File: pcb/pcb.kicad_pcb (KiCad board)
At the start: 4 copper layers, 71.5 x 115.4 mm, 173 parts, among them J1 AudioJack3_SwitchTR, J100 Conn_02x05_Odd_Even, J102 Conn_01x03, J500 FPC_18P_1.0MM, J600 USB_B_Micro, Q300 IRLML6402, SW1 SW_SP3T, SW700 SW_Push, SW701 SW_Push, SW702 SW_Push, SW703 SW_Push, SW704 SW_Push, SW705 SW_Push, SW706 SW_Push, SW707 SW_Push, U1 LTC3456, U100 LPC5500, U400 CS43130, U401 ADP150-3.0, U402 ADP150-1.8, U403 ADP150-1.8, U404 SN74AVC4T245PW, U405 PCA9306, U501 LT1617, U502 LM324, U600 USBLC6-2SC6, Y1 32.768kHz, Y2 24MHz, Y400 22.5792MHz

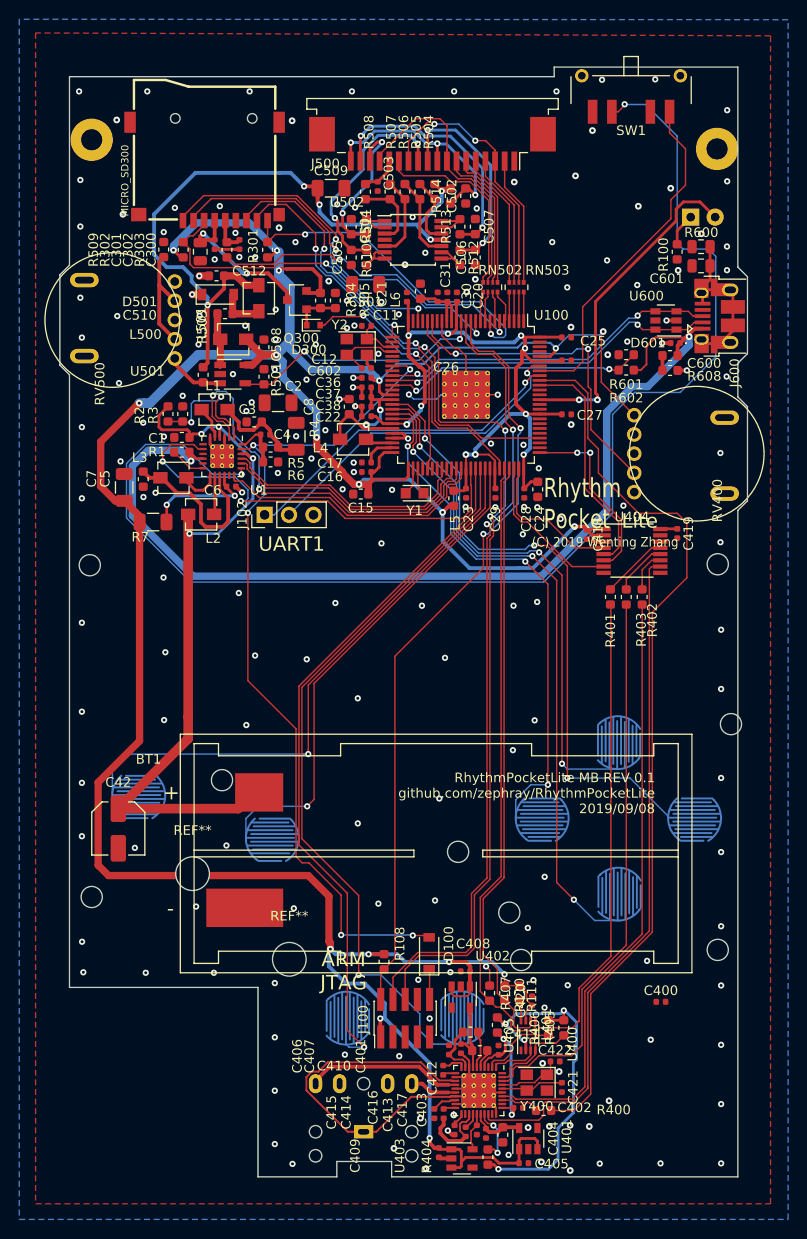
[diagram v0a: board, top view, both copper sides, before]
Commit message: rev 0.1
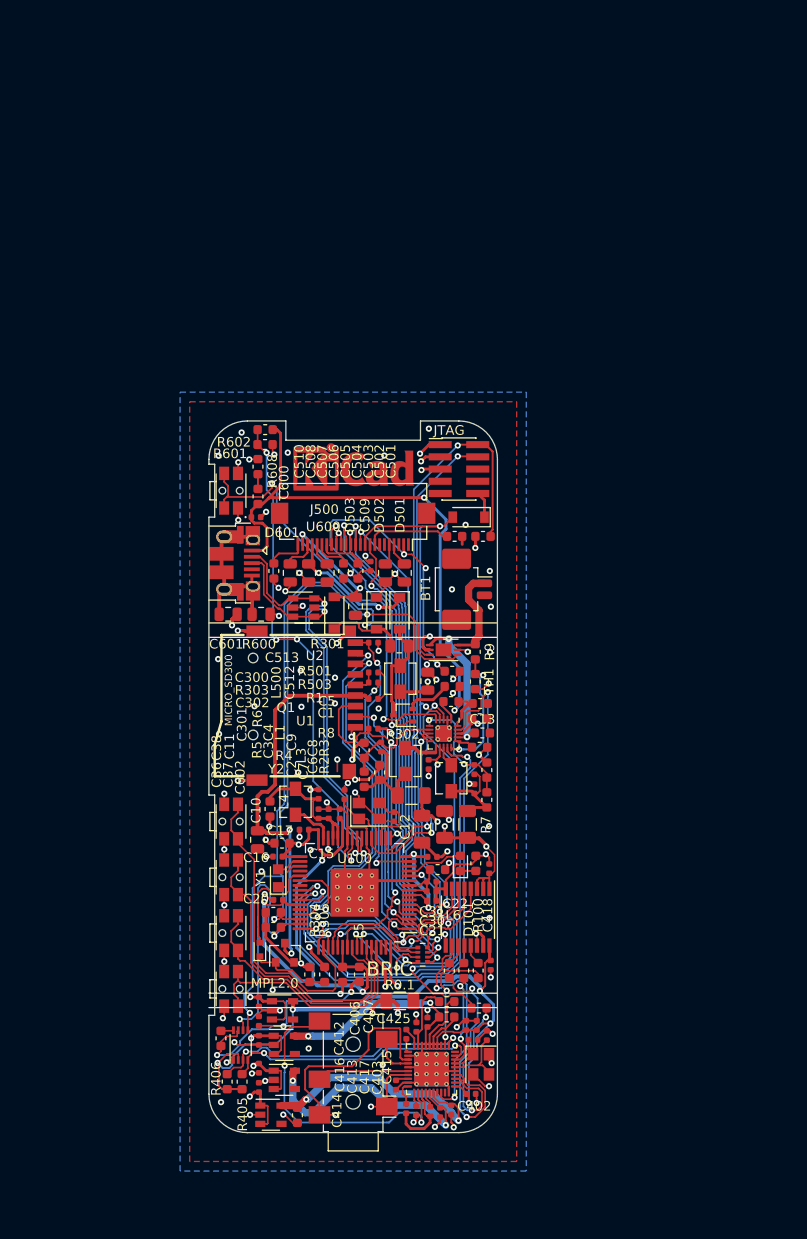
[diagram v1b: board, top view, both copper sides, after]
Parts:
- removed C23, C25, C26, C27, C28, C29: 100nF, Capacitor_SMD:C_0402_1005Metric
- removed C42: 100uF, Capacitor_SMD:C_Elec_5x5.4
- removed G***: LOGO, footprints:logo
- removed J102: Conn_01x03, Connector_PinHeader_2.54mm:PinHeader_1x03_P2.54mm_Vertical
- removed L2: 4.7uH, Inductor_SMD:L_Vishay_IHLP-1212
- removed L401: 120R, Inductor_SMD:L_0603_1608Metric
- removed L501: 22uH, Inductor_SMD:L_Vishay_IHLP-1212
- removed R404, R504, R505, R507, R508: 10K, Resistor_SMD:R_0603_1608Metric
- removed R506: 75K, Resistor_SMD:R_0603_1608Metric
- removed R509: 20K, Resistor_SMD:R_0603_1608Metric
- removed R510, R511, R512, R513, R514: 33, Resistor_SMD:R_0603_1608Metric
- removed the REF** at (128.3, 127.1)
- removed the REF** at (184.3, 111.5)
- removed the REF** at (182.8, 51.7)
- removed the REF** at (117.8, 50.8)
- removed the REF** at (131.4, 117.3)
- removed the REF** at (117.6, 95.0)
- removed the REF** at (138.4, 136.0)
- removed the REF** at (182.9, 94.9)
- removed the REF** at (117.8, 129.5)
- removed the REF** at (182.9, 135.0)
- removed the REF** at (155.9, 124.8)
- removed the REF** at (162.5, 136.1)
- removed the REF** at (161.2, 131.1)
- removed RN502: 33R, Resistor_SMD:R_Array_Convex_4x0402
- removed RV400: RK14J11A0A02, footprints:Potentiometer_RK14J
- removed RV500: RK14J11A0A02/50K, footprints:Potentiometer_RK14J
- removed SW700, SW705, SW706, SW707: SW_Push, footprints:contact
- removed U501: LT1617, Package_TO_SOT_SMD:TSOT-23-5
- removed U502: LM324, Package_SO:TSSOP-14_4.4x5mm_P0.65mm
- added C10: 22uF, Capacitor_SMD:C_0603_1608Metric, F.Cu at (136.3, 120.3)
- added C13: 10uF, Capacitor_SMD:C_0603_1608Metric, F.Cu at (158.4, 112.4)
- added C424: 1uF, Capacitor_SMD:C_0402_1005Metric, F.Cu at (135.2, 140.4)
- added C425: 100uF, Capacitor_SMD:C_1206_3216Metric, F.Cu at (149.8, 140.3)
- added C513: 4.7uF/25V, Capacitor_SMD:C_0805_2012Metric, F.Cu at (149.8, 103.4)
- added C9: 2.2uF, Capacitor_SMD:C_0402_1005Metric, F.Cu at (152.8, 115.7)
- added D502: MBR0530, Diode_SMD:D_SOD-123, F.Cu at (147.4, 100.0)
- added D503: MBR0530, Diode_SMD:D_SOD-123, F.Cu at (143.0, 99.9)
- added Q1: Q_NMOS_GSD, Package_TO_SOT_SMD:SOT-323_SC-70, F.Cu at (150.2, 110.6)
- added R502: 10K, Resistor_SMD:R_0603_1608Metric, F.Cu at (155.6, 92.0)
- added R8: 1.87K, Resistor_SMD:R_0603_1608Metric, F.Cu at (158.2, 113.9)
- added R9: 100K, Resistor_SMD:R_0603_1608Metric, F.Cu at (157.7, 104.0)
- added REF**: KiCad-Logo_5mm_SilkScreen, Symbol:KiCad-Logo_5mm_SilkScreen, B.Cu at (145.0, 147.4)
- added REF**: KiCad-Logo_5mm_Copper, Symbol:KiCad-Logo_5mm_Copper, F.Cu at (145.1, 85.3)
- added TH1: 100K, Resistor_SMD:R_0603_1608Metric, F.Cu at (157.7, 107.1)
- added U2: LTC2942-1, Package_DFN_QFN:DFN-6-1EP_3x2mm_P0.5mm_EP1.65x1.35mm, F.Cu at (154.4, 103.8)
- added U406: ADP150-1.8, Package_TO_SOT_SMD:SOT-23-5, F.Cu at (137.7, 141.3)
- BT1: value Battery -> Molex1.25; footprint footprints:BatteryHolder_Keystone_5204_5226 -> Connector_Molex:Molex_PicoBlade_53261-0271_1x02-1MP_P1.25mm_Horizontal
- C1: value 4.7uF -> 10uF
- C5: value 22uF -> 10uF
- C501, C509: value 22uF/25V -> 4.7uF/25V; footprint Capacitor_SMD:C_1206_3216Metric -> Capacitor_SMD:C_0805_2012Metric
- C502, C506, C507: value 4.7uF -> 4.7uF/25V; footprint Capacitor_SMD:C_0603_1608Metric -> Capacitor_SMD:C_0805_2012Metric
- C504, C505: value 4.7uF -> 1uF
- C508: value 10uF -> 4.7uF/25V; footprint Capacitor_SMD:C_0603_1608Metric -> Capacitor_SMD:C_0805_2012Metric
- C510: value 220nF -> 1uF
- C512: footprint Capacitor_SMD:C_0603_1608Metric -> Capacitor_SMD:C_0805_2012Metric
- C8: value 22uF -> 220pF; footprint Capacitor_SMD:C_0603_1608Metric -> Capacitor_SMD:C_0402_1005Metric
- D101: footprint LED_THT:LED_D5.0mm -> LED_SMD:LED_0603_1608Metric; moved to F.Cu
- J1: value AudioJack3_SwitchTR -> AudioJack3_SwitchDualS; footprint footprints:Jack_3.5mm_PJ307C -> footprints:Jack_3.5mm_PJ327E_5A; moved to F.Cu
- J500: value FPC_18P_1.0MM -> FH12A-24S-0.5SH; footprint Connector_FFC-FPC:TE_1-84953-8_1x18-1MP_P1.0mm_Horizontal -> Connector_FFC-FPC:Hirose_FH12-24S-0.5SH_1x24-1MP_P0.50mm_Horizontal
- L3: value 10uH -> 4.7uH
- L500: value 22uH -> 10uH
- R2: value 100K -> 2.05M
- R3: value 80.6K -> 649K
- R301, R302, R303: footprint Resistor_SMD:R_0603_1608Metric -> Resistor_SMD:R_0402_1005Metric
- R5: value 100K -> 1M
- R503: value 330K -> 3R
- SW1: value SW_SP3T -> SW_Push; footprint footprints:SW_SP3T_JSM0701SAQNL -> Button_Switch_SMD:SW_SPST_EVQP7C
- SW701, SW702, SW703, SW704: footprint footprints:contact -> Button_Switch_SMD:SW_SPST_EVQP7C; moved to F.Cu
- U1: value LTC3456 -> LTC3554; footprint Package_DFN_QFN:VQFN-24-1EP_4x4mm_P0.5mm_EP2.45x2.45mm_ThermalVias -> Package_DFN_QFN:VQFN-20-1EP_3x3mm_P0.4mm_EP1.7x1.7mm_ThermalVias
- U100: value LPC5500 -> LPC5500_FBD64; footprint Package_QFP:TQFP-100-1EP_14x14mm_P0.5mm_EP5x5mm_ThermalVias -> Package_QFP:LQFP-64-1EP_10x10mm_P0.5mm_EP5x5mm_ThermalVias
- U401: value ADP150-3.0 -> ADP150-3.3
- Y1: value 32.768kHz -> DNP/32.768kHz
- moved D101 71.3 mm to (156.2, 126.0), turned to 90 degrees
- moved RN503 70.1 mm to (152.2, 135.5), turned to 0 degrees
- moved R304 70.1 mm to (140.5, 137.6)
- moved R305 70.1 mm to (142.0, 137.6)
- moved Q300 67.9 mm to (137.9, 135.3), turned to 90 degrees
- moved R100 66.9 mm to (157.8, 126.0), turned to 90 degrees
- moved C20 65.4 mm to (137.2, 129.8), turned to 180 degrees
- moved D300 65.2 mm to (135.3, 134.9), turned to 90 degrees
- moved C21 62.8 mm to (153.2, 129.9), turned to 0 degrees
- moved C30 61.8 mm to (153.2, 128.9), turned to 0 degrees
- moved C301 61.4 mm to (135.1, 123.5)
- moved C601 61.1 mm to (132.0, 100.1), turned to 0 degrees
- moved C31 60.8 mm to (153.2, 127.9), turned to 0 degrees
- moved L6 60.2 mm to (153.8, 126.7), turned to 180 degrees
- moved R600 59.6 mm to (135.4, 100.1), turned to 0 degrees
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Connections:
- C1 pad 1: +BATT -> GND
- C1 pad 2: GND -> +SYS
- C2 pad 1: +1V8 -> +2V0
- C36 pad 1: Net-(C36-Pad1) -> Net-(C10-Pad1)
- C37 pad 1: Net-(C36-Pad1) -> Net-(C10-Pad1)
- C38 pad 1: Net-(C36-Pad1) -> Net-(C10-Pad1)
- C400 pad 1: Net-(C400-Pad1) -> +1V8
- C401 pad 1: Net-(C400-Pad1) -> +1V8
- C402 pad 1: Net-(C400-Pad1) -> +1V8
- C405 pad 1: Net-(C405-Pad1) -> +SYS
- C408 pad 1: Net-(C405-Pad1) -> +2V0
- C409 pad 1: Net-(C405-Pad1) -> +2V0
- C5 pad 1: Net-(C5-Pad1) -> VBUS
- C501 pad 1: Net-(C501-Pad1) -> GND
- C501 pad 2: GND -> Net-(C501-Pad2)
- C502 pad 2: /lcd/LCD_V5 -> Net-(C502-Pad2)
- C504 pad 2: /lcd/LCD_V1 -> Net-(C504-Pad2)
- C505 pad 2: /lcd/LCD_V2 -> Net-(C505-Pad2)
- C506 pad 2: /lcd/LCD_V3 -> Net-(C506-Pad2)
- C507 pad 2: /lcd/LCD_V4 -> /lcd/PREVGH
- C508 pad 1: +3V3 -> Net-(C508-Pad1)
- C509 pad 1: Net-(C501-Pad1) -> /lcd/PREVGL
- C510 pad 2: Net-(C510-Pad2) -> GND
- C512 pad 2: Net-(C501-Pad1) -> +3V3
- C8 pad 1: Net-(C36-Pad1) -> Net-(C6-Pad1)
- C8 pad 2: GND -> Net-(C8-Pad2)
- D501 pad 1: GND -> /lcd/PREVGH
- D501 pad 2: Net-(C510-Pad1) -> Net-(C513-Pad1)
- J500 pad 1: GND -> Net-(J500-Pad1)
- J500 pad 10: /lcd/LCD_V3 -> POR
- J500 pad 11: /lcd/LCD_V2 -> /lcd/EPD_RS
- J500 pad 12: /lcd/LCD_CPL -> /lcd/EPD_CS
- J500 pad 13: /lcd/LCD_S -> /lcd/EPD_SCLK
- J500 pad 14: +3V3 -> /lcd/EPD_SDI
- J500 pad 15: /lcd/LCD_FR -> +3V3
- J500 pad 16: /lcd/LCD_V1 -> +3V3
- J500 pad 17: /lcd/LCD_V4 -> GND
- J500 pad 18: /lcd/LCD_V5 -> Net-(C504-Pad2)
- J500 pad 2: /lcd/LCD_CPG -> /lcd/GDR
- J500 pad 3: /lcd/LCD_CPL -> /lcd/RESE
- J500 pad 4: /lcd/LCD_ST -> Net-(C501-Pad2)
- J500 pad 5: /lcd/LCD_D0 -> Net-(C502-Pad2)
- J500 pad 6: /lcd/LCD_D1 -> Net-(J500-Pad6)
- J500 pad 7: /lcd/LCD_CP -> Net-(J500-Pad7)
- J500 pad 8: /lcd/LCD_FR -> Net-(J500-Pad8)
- J500 pad 9: /lcd/LCD_V5 -> EPD_BUSY
- L3 pad 1: Net-(C5-Pad1) -> Net-(L3-Pad1)
- L3 pad 2: Net-(L3-Pad2) -> Net-(C6-Pad1)
- L4 pad 2: Net-(C36-Pad1) -> Net-(C10-Pad1)
- L500 pad 2: Net-(C510-Pad2) -> Net-(C513-Pad1)
- R2 pad 1: Net-(R2-Pad1) -> Net-(C8-Pad2)
- R2 pad 2: +BATT -> Net-(C6-Pad1)
- R3 pad 2: Net-(R2-Pad1) -> Net-(C8-Pad2)
- R4 pad 2: +1V8 -> +2V0
- R501 pad 1: ~LCD_PWR_EN -> /lcd/GDR
- R503 pad 2: Net-(C501-Pad1) -> GND
- RN503 pad 1: STN_D0 -> EPD_DC
- RN503 pad 2: STN_ST -> SPI_SSEL0
- RN503 pad 3: STN_CPL -> SPI_SCK
- RN503 pad 4: STN_CPG -> SPI_MOSI
- RN503 pad 5: /lcd/LCD_CPG -> /lcd/EPD_SDI
- RN503 pad 6: /lcd/LCD_CPL -> /lcd/EPD_SCLK
- RN503 pad 7: /lcd/LCD_ST -> /lcd/EPD_CS
- RN503 pad 8: /lcd/LCD_D0 -> /lcd/EPD_RS
- SW1 pad 1: HOLD -> GND
- SW1 pad 2: Net-(SW1-Pad2) -> /power/PWR_KEY
- SW701 pad 1: SW_ST -> SW_UP
- SW702 pad 1: SW_A -> SW_LE
- SW703 pad 1: SW_B -> SW_DN
- SW704 pad 1: SW_UP -> SW_RI
- U1 pad 1: Net-(R2-Pad1) -> Net-(R1-Pad1)
- U1 pad 10: VBUS -> STBY
- U1 pad 11: Net-(U1-Pad11) -> Net-(L1-Pad2)
- U1 pad 12: Net-(R1-Pad1) -> +SYS
- U1 pad 13: Net-(L3-Pad2) -> Net-(L3-Pad1)
- U1 pad 14: Net-(L2-Pad2) -> CHRG
- U1 pad 15: Net-(C5-Pad1) -> Net-(R9-Pad1)
- U1 pad 16: Net-(C6-Pad1) -> Net-(R8-Pad2)
- U1 pad 18: USB_SUSPEND -> +SYS
- U1 pad 19: /power/PWR_KEY -> USB_SUSPEND
- U1 pad 2: BAT_LOW -> GND
- U1 pad 20: PB_STAT -> VBUS
- U1 pad 21: PMIC_ON_REQ -> GND
- U1 pad 3: GND -> PB_STAT
- U1 pad 4: +BATT -> POR
- U1 pad 5: Net-(L1-Pad2) -> /power/PWR_KEY
- U1 pad 6: GND -> Net-(C8-Pad2)
- U1 pad 7: Net-(U1-Pad7) -> Net-(C4-Pad2)
- U1 pad 8: EXT_PWR_GOOD -> PMIC_ON_REQ
- U1 pad 9: Net-(U1-Pad9) -> PMIC_ON_REQ
- U100 pad 1: STN_CPG -> SD0_CLK
- U100 pad 10: STN_S -> Net-(C30-Pad1)
- U100 pad 11: SD0_D3 -> GND
- U100 pad 12: /cpu/MPU_JTAG_TMS -> SAI1_MCLK
- U100 pad 13: /cpu/MPU_JTAG_TCK -> /cpu/LED
- U100 pad 14: ~LCD_PWR_EN -> Net-(U100-Pad14)
- U100 pad 15: Net-(C20-Pad1) -> SD0_D2
- U100 pad 16: Net-(C30-Pad1) -> Net-(C20-Pad1)
- U100 pad 17: Net-(C30-Pad1) -> SD0_CMD
- U100 pad 18: GND -> PMIC_ON_REQ
- U100 pad 19: GND -> Net-(C12-Pad1)
- U100 pad 2: STN_CPL -> EPD_DC
- U100 pad 20: ADC1_IN0 -> Net-(C11-Pad1)
- U100 pad 21: /cpu/MPU_JTAG_TDO -> POR
- U100 pad 22: Net-(U100-Pad22) -> GND
- U100 pad 23: SD0_D2 -> /usb/USB_DP
- U100 pad 24: Net-(U100-Pad24) -> /usb/USB_DM
- U100 pad 25: Net-(C20-Pad1) -> Net-(R601-Pad2)
- U100 pad 26: SD0_CMD -> GND
- U100 pad 27: Net-(U100-Pad27) -> +3V3
- U100 pad 28: Net-(C11-Pad1) -> Net-(C10-Pad1)
- U100 pad 29: Net-(C12-Pad1) -> Net-(C10-Pad1)
- U100 pad 3: STN_ST -> ~SD0_CD
- U100 pad 30: Net-(U100-Pad30) -> GND
- U100 pad 31: Net-(U100-Pad31) -> Net-(L4-Pad1)
- U100 pad 32: POR -> +3V3
- U100 pad 33: GND -> +3V3
- U100 pad 34: /usb/USB_DP -> Net-(U100-Pad34)
- U100 pad 35: /usb/USB_DM -> Net-(U100-Pad35)
- U100 pad 36: Net-(R601-Pad2) -> Net-(U100-Pad36)
- U100 pad 37: GND -> ~SD0_PWR_EN
- U100 pad 38: +3V3 -> CODEC_RST
- U100 pad 39: Net-(C36-Pad1) -> Net-(U100-Pad39)
- U100 pad 4: STN_D0 -> SD0_D3
- U100 pad 40: SW_LE -> USB_SUSPEND
- U100 pad 41: SW_UP -> CHRG
- U100 pad 42: SW_DN -> PB_STAT
- U100 pad 43: SW_RI -> Net-(C20-Pad1)
- U100 pad 44: Net-(C20-Pad1) -> Net-(U100-Pad44)
- U100 pad 45: Net-(C36-Pad1) -> SD0_D0
- U100 pad 46: GND -> I2C1_SDA
- U100 pad 47: GND -> I2C1_SCL
- U100 pad 48: Net-(L4-Pad1) -> SAI1_TXD
- U100 pad 49: +3V3 -> SAI1_TXC
- U100 pad 5: STN_D1 -> /cpu/MPU_JTAG_TMS
- U100 pad 50: +3V3 -> SW_UP
- U100 pad 51: +3V3 -> SD0_D1
- U100 pad 52: Net-(U100-Pad52) -> EPD_BUSY
- U100 pad 53: Net-(U100-Pad53) -> SPI_MOSI
- U100 pad 54: Net-(U100-Pad54) -> Net-(C20-Pad1)
- U100 pad 55: ~SD0_PWR_EN -> SPI_SSEL0
- U100 pad 56: Net-(U100-Pad56) -> SW_LE
- U100 pad 57: Net-(U100-Pad57) -> SPI_SCK
- U100 pad 58: PMIC_ON_REQ -> SAI1_TXFS
- U100 pad 59: Net-(U100-Pad59) -> SW_DN
- U100 pad 6: SD0_CLK -> /cpu/MPU_JTAG_TCK
- U100 pad 60: PB_STAT -> SW_RI
- U100 pad 61: BAT_LOW -> +3V3
- U100 pad 62: USB_SUSPEND -> Net-(U100-Pad62)
- U100 pad 63: Net-(C20-Pad1) -> Net-(U100-Pad63)
- U100 pad 64: EXT_PWR_GOOD -> GND
- U100 pad 65: SW_ST -> GND
- U100 pad 7: STN_CP -> Net-(U100-Pad7)
- U100 pad 8: ~SD0_CD -> Net-(C20-Pad1)
- U100 pad 9: STN_FR -> Net-(C30-Pad1)
- U400 pad 14: Net-(J1-PadT) -> Net-(J1-Pad2)
- U400 pad 16: Net-(J1-PadR) -> Net-(J1-Pad3)
- U400 pad 22: Net-(U400-Pad22) -> Net-(J1-Pad5)
- U400 pad 31: Net-(C400-Pad1) -> +1V8
- U400 pad 4: Net-(C400-Pad1) -> +1V8
- U401 pad 1: Net-(C405-Pad1) -> +SYS
- U401 pad 3: Net-(C405-Pad1) -> +SYS
- U402 pad 1: Net-(C405-Pad1) -> +2V0
- U402 pad 3: Net-(C405-Pad1) -> +2V0
- U403 pad 1: Net-(C405-Pad1) -> +2V0
- U403 pad 3: Net-(C405-Pad1) -> +2V0
- Y1 pad 1: Net-(U100-Pad53) -> Net-(U100-Pad35)
- Y1 pad 2: Net-(U100-Pad52) -> Net-(U100-Pad34)
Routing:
- net +3V3: track 359.5 -> 84.8 mm, vias 19 -> 16
- net GND: track 104.4 -> 214.5 mm, vias 185 -> 103
- net /power/PWR_KEY: track 135.0 -> 46.5 mm
- net /cpu/MPU_JTAG_TDO: track 85.1 -> 0.00 mm, vias 2 -> 0
- net +SYS: track 0.00 -> 82.3 mm, vias 0 -> 5
- net SW_SE: track 77.5 -> 0.00 mm, vias 1 -> 0
- net SW_ST: track 72.5 -> 0.00 mm, vias 1 -> 0
- net +2V0: track 0.00 -> 72.0 mm, vias 0 -> 4
- net +BATT: track 81.5 -> 10.2 mm, vias 4 -> 0
- net Net-(C501-Pad1): track 70.6 -> 0.00 mm, vias 5 -> 0
- net SAI1_MCLK: track 94.0 -> 25.4 mm, vias 0 -> 2
- net SW_A: track 61.1 -> 0.00 mm, vias 1 -> 0
- net /lcd/EPD_SDI: track 0.00 -> 53.1 mm, vias 0 -> 2
- net SW_B: track 52.2 -> 0.00 mm, vias 1 -> 0
- net /lcd/EPD_CS: track 0.00 -> 51.6 mm, vias 0 -> 2
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- removed copper zone on In1.Cu, net Net-(C20-Pad1)
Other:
- board size 71.5 x 115.4 mm -> 30 x 74 mm
- net class USB: clearance 0.2032 -> 0.1524; trace_width 0.1524 -> 0.18
- board text added: "2.13 EINK"
- board text added: "2Vrms"
- board text added: "40nm"
- board text added: "ARM"
- board text added: "Analog Devices"
- board text added: "BRIC"
- board text added: "Bric"
- board text added: "Cirrus Logic"
- board text added: "Cortex-M33"
- board text added: "E-ink"
- board text added: "FreeRTOS FatFs OpenSDA"
- board text added: "JTAG"
- board text added: "Linear Technology"
- board text added: "MPL2.0"
- board text added: "MasterHiFi"
- board text added: "NXP"
- board text added: "Open Source Hardware"
- board text added: "PowerPath"
- board text added: "R0.1"
- board text added: "VFPv5"
- board text added: "eNVM"
- board text removed: "(C) 2019 Wenting Zhang"
- board text removed: "ARM JTAG"
- board text removed: "Lite"
- board text removed: "Rhythm Pocket"
- board text removed: "RhythmPocketLite MB REV 0.1 github.com/zephray/RhythmPocketLite 2019/09/08"
- board text removed: "UART1"
